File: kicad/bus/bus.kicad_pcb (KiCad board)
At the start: 2 copper layers, 45 parts, among them J1 Barrel_Jack, U29 L7805

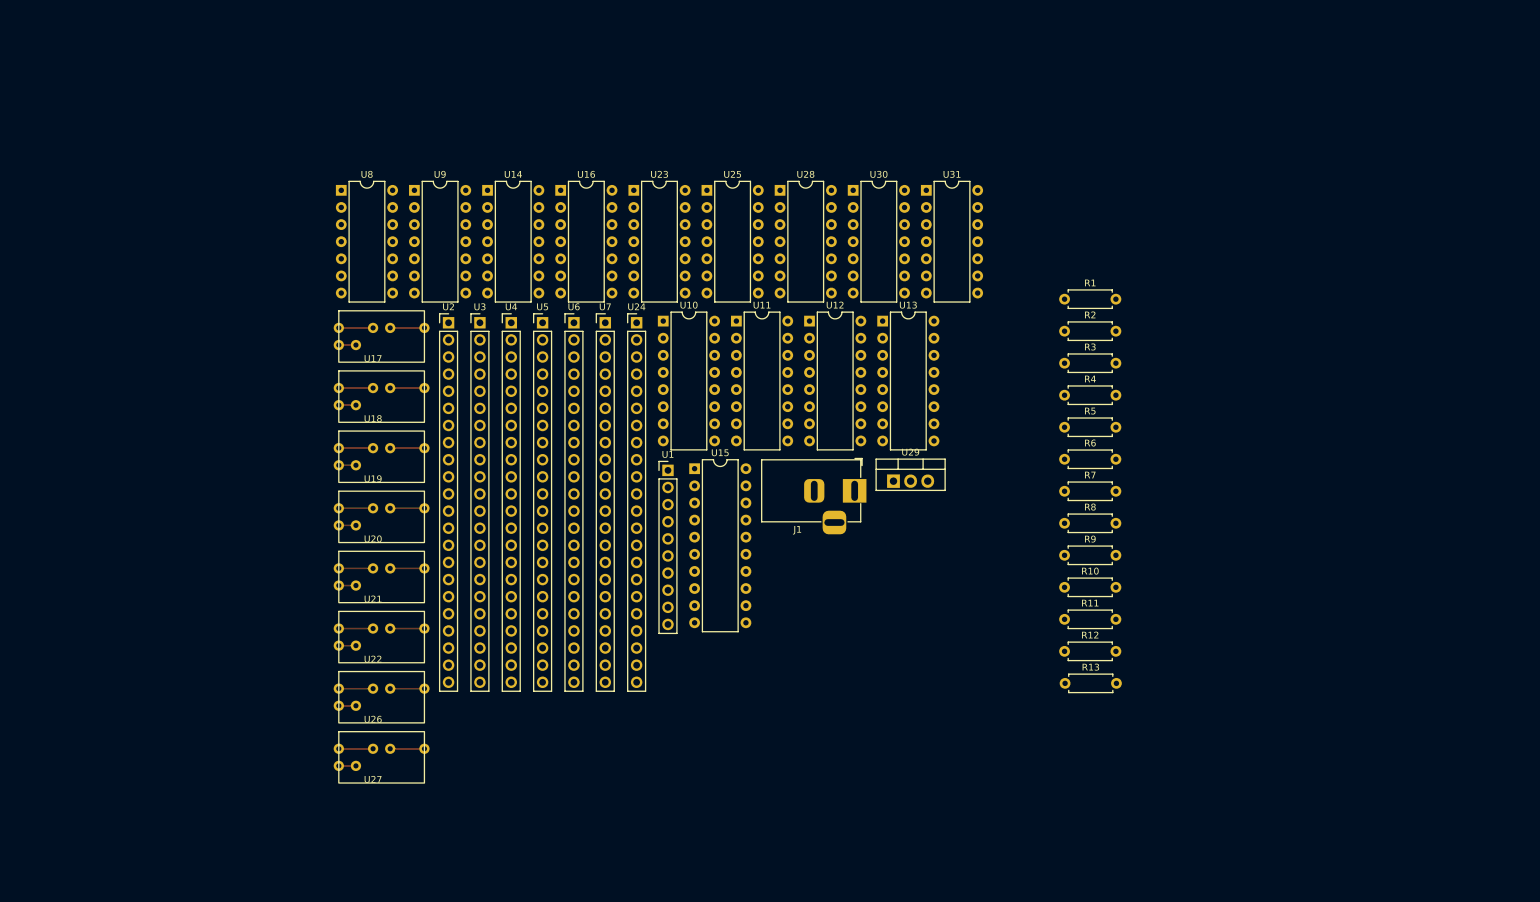
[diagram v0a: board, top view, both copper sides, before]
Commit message: stuff
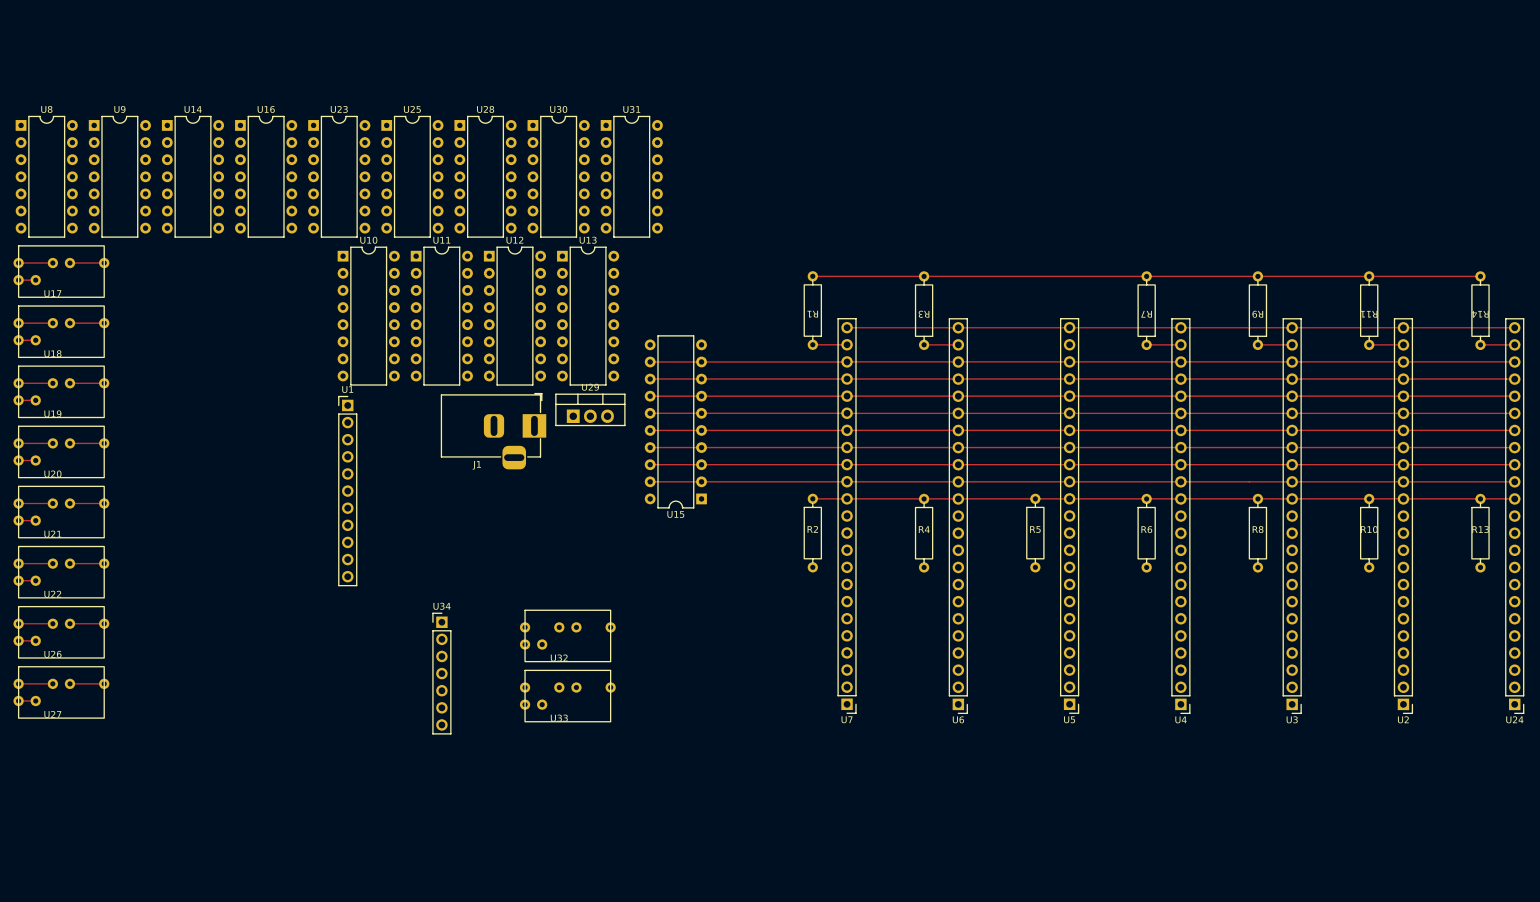
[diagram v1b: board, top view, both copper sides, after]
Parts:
- removed R12: 1k, Resistor_THT:R_Axial_DIN0207_L6.3mm_D2.5mm_P7.62mm_Horizontal
- added R14: 1k, custom_footprint_library:0.4_pitch_resistor, F.Cu at (270.5, 76.2)
- added U32: ~, custom_footprint_library:jumper, F.Cu at (133.8, 128.3)
- added U33: ~, custom_footprint_library:jumper, F.Cu at (133.8, 137.2)
- added U34: ~, Connector_PinHeader_2.54mm:PinHeader_1x07_P2.54mm_Vertical, F.Cu at (116.4, 122.4)
- R1, R10, R11, R13, R2, R3, R4, R5, R6, R7, R8, R9: footprint Resistor_THT:R_Axial_DIN0207_L6.3mm_D2.5mm_P7.62mm_Horizontal -> custom_footprint_library:0.4_pitch_resistor
- U1: footprint Connector_PinHeader_2.54mm:PinHeader_1x10_P2.54mm_Vertical -> Connector_PinHeader_2.54mm:PinHeader_1x11_P2.54mm_Vertical
- U2, U24, U3, U4, U5, U6, U7: footprint Connector_PinHeader_2.54mm:PinHeader_1x22_P2.54mm_Vertical -> Connector_PinHeader_2.54mm:PinHeader_1x23_P2.54mm_Vertical
- moved U2 152.6 mm to (259.1, 134.6), turned to 180 degrees
- moved U24 142.1 mm to (275.6, 134.6), turned to 180 degrees
- moved U3 133.1 mm to (242.6, 134.6), turned to 180 degrees
- moved U4 114.4 mm to (226.1, 134.6), turned to 180 degrees
- moved U5 96.5 mm to (209.6, 134.6), turned to 180 degrees
- moved U6 80.4 mm to (193.0, 134.6), turned to 180 degrees
- moved U7 67.0 mm to (176.5, 134.6), turned to 180 degrees
- moved R13 65.5 mm to (270.5, 109.2)
- moved R11 64.3 mm to (254.0, 76.2), turned to 180 degrees
- moved U1 48.5 mm to (102.5, 90.3)
- moved U11 48.5 mm to (112.6, 68.1)
- moved U25 48.5 mm to (108.2, 48.7)
- moved U28 48.5 mm to (119.1, 48.7)
- moved U9 48.5 mm to (64.8, 48.7)
- moved U8 48.5 mm to (54.0, 48.7)
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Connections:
- U16 pad 4: Net-(U10-GND) -> Net-(U16-2A)
- U16 pad 5: Net-(U10-GND) -> Net-(U16-2B)
- U16 pad 6: unconnected-(U16-2Q-Pad6) -> Net-(U16-2Q)
- U20 pad 1: Net-(U20-IN) -> Net-(U16-2Q)
- U21 pad 1: Net-(U19-IN) -> Net-(U21-IN)
- U28 pad 13: Net-(U19-IN) -> Net-(U21-IN)
- U30 pad 4: Net-(U10-GND) -> Net-(U21-IN)
- U30 pad 5: Net-(U10-GND) -> Net-(U16-2B)
- U30 pad 6: unconnected-(U30-2Q-Pad6) -> Net-(U19-IN)
- U31 pad 1: Net-(U20-IN) -> Net-(U16-2A)
- U31 pad 9: Net-(U19-IN) -> Net-(U21-IN)
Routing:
- net Net-(U10-GND): track 0.00 -> 203.2 mm
- net Net-(U15-D5): track 0.00 -> 128.3 mm
- net Net-(U15-D3): track 0.00 -> 128.3 mm
- net Net-(U15-D7): track 0.00 -> 128.3 mm
- net Net-(U15-D6): track 0.00 -> 128.3 mm
- net Net-(U15-D4): track 0.00 -> 128.3 mm
- net Net-(U15-D2): track 0.00 -> 128.3 mm
- net Net-(U15-D1): track 0.00 -> 128.3 mm
- net Net-(U15-D0): track 0.00 -> 128.3 mm
- net Net-(U16-2B): track 0.00 -> 99.1 mm
- net Net-(U7-FAULT): track 0.00 -> 5.08 mm
- net Net-(U4-FAULT): track 0.00 -> 5.08 mm
- net Net-(U6-FAULT): track 0.00 -> 5.08 mm
- net Net-(U3-FAULT): track 0.00 -> 5.08 mm
- net Net-(U24-FAULT): track 0.00 -> 5.08 mm
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
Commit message: Finished main PCB design
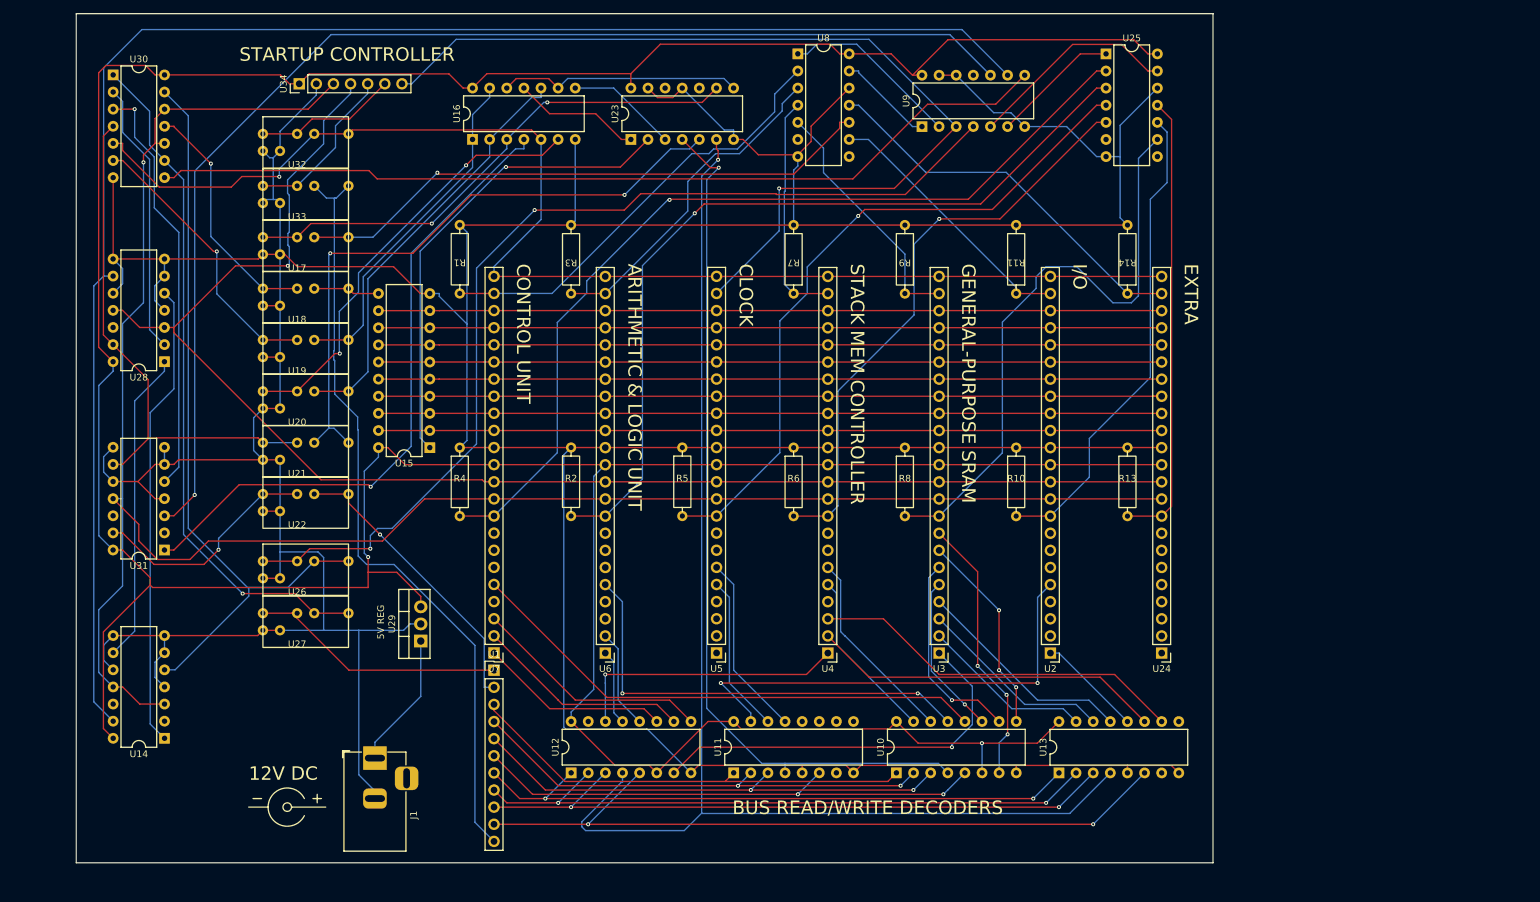
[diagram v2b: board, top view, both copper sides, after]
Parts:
- moved U9 122.8 mm to (187.6, 48.9), turned to 90 degrees
- moved U8 115.7 mm to (169.2, 38.1)
- moved U10 112.3 mm to (183.9, 144.8), turned to 90 degrees
- moved U25 107.3 mm to (215.0, 38.1)
- moved U13 106.3 mm to (208.0, 144.8), turned to 90 degrees
- moved U14 90.9 mm to (75.3, 139.7), turned to 180 degrees
- moved U31 90.9 mm to (75.3, 111.7), turned to 180 degrees
- moved U11 90.0 mm to (159.7, 144.8), turned to 90 degrees
- moved U33 84.0 mm to (94.9, 62.8)
- moved U32 82.9 mm to (94.9, 55.0)
- moved U34 82.6 mm to (95.2, 42.5), turned to 90 degrees
- moved U12 77.6 mm to (135.6, 144.8), turned to 90 degrees
- moved R4 69.3 mm to (119.1, 101.6)
- moved U30 62.7 mm to (67.6, 41.2)
- moved U28 56.1 mm to (75.3, 83.8), turned to 180 degrees
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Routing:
- net Net-(U10-GND): track 203.2 -> 822.5 mm
- net Net-(U10-E1): track 0.00 -> 588.7 mm, vias 0 -> 2
- net Net-(U14-0CLK): track 0.00 -> 293.3 mm, vias 0 -> 1
- net Net-(U14-1Q): track 0.00 -> 239.4 mm
- net Net-(U2-CLK_B): track 0.00 -> 218.6 mm, vias 0 -> 1
- net Net-(U12-E2#): track 0.00 -> 193.9 mm, vias 0 -> 1
- net Net-(U31-0CLK): track 0.00 -> 182.8 mm, vias 0 -> 1
- net Net-(U26-IN): track 0.00 -> 148.6 mm, vias 0 -> 2
- net Net-(U34-FAULT): track 0.00 -> 139.8 mm, vias 0 -> 1
- net Net-(U25-A0): track 0.00 -> 135.6 mm, vias 0 -> 1
- net Net-(U30-4Q): track 0.00 -> 134.9 mm
- net Net-(U10-E2#): track 0.00 -> 129.2 mm, vias 0 -> 1
- net Net-(U25-A1): track 0.00 -> 124.3 mm, vias 0 -> 1
- net Net-(U1-Start): track 0.00 -> 114.4 mm
- net Net-(U14-0D): track 0.00 -> 113.5 mm
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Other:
- board outline added: 168.7 x 126 mm
- board text added: "12V DC"
- board text added: "5V REG"
- board text added: "ARITHMETIC & LOGIC UNIT"
- board text added: "BUS READ/WRITE DECODERS"
- board text added: "CLOCK"
- board text added: "CONTROL UNIT"
- board text added: "EXTRA"
- board text added: "GENERAL-PURPOSE SRAM"
- board text added: "I/O"
- board text added: "STACK MEM CONTROLLER"
- board text added: "STARTUP CONTROLLER"

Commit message: Working on clock
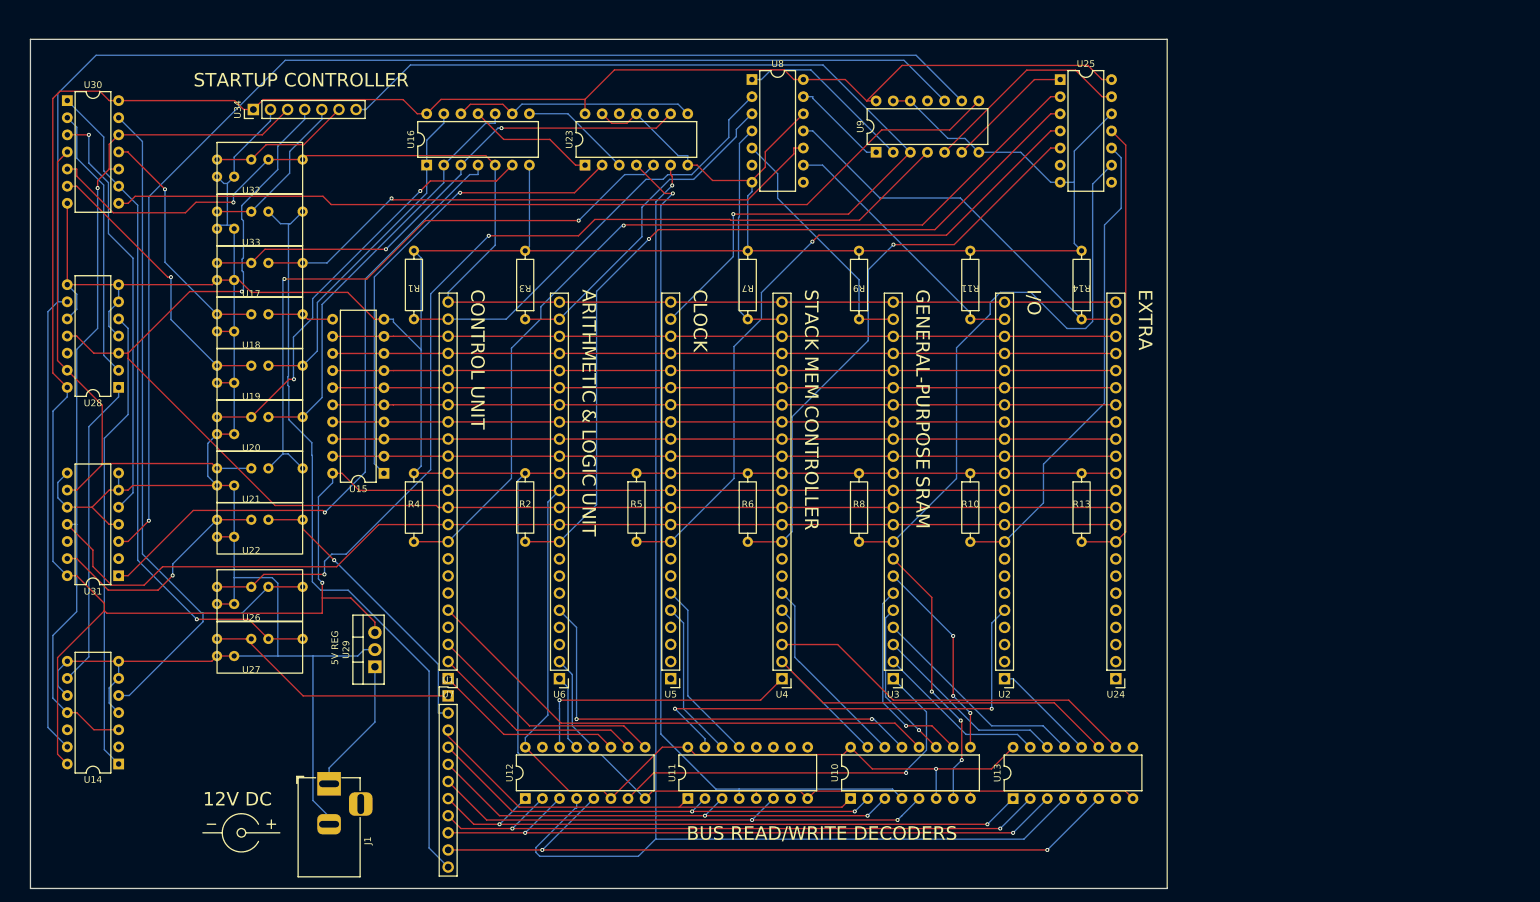
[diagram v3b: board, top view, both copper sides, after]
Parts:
- moved R2 7.80 mm to (128.8, 105.4)
- moved R3 7.80 mm to (128.8, 72.4)
- moved R8 7.80 mm to (178.3, 105.4)
- moved R9 7.80 mm to (178.3, 72.4)
- moved U11 7.80 mm to (152.9, 148.6)
- moved U23 7.80 mm to (137.7, 54.6)
- moved U24 7.80 mm to (216.4, 130.8)
- moved U25 7.80 mm to (208.2, 41.9)
- moved U4 7.80 mm to (166.9, 130.8)
- moved U9 7.80 mm to (180.8, 52.7)
- moved U29 7.80 mm to (106.5, 129.0)
- moved U7 7.80 mm to (117.3, 130.8)
- moved U1 7.80 mm to (117.3, 133.4)
- moved U14 7.80 mm to (68.5, 143.5)
- moved U15 7.80 mm to (107.8, 100.3)
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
